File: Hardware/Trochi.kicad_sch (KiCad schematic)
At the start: 49 parts, among them IC1 ICM-42688-P, J1 JST PH, J2 JST-SH, J3 JST-SH, J4 JST-SH, J5 JST-SH, J6 JST_SH, Q1 AO3400A, Q2 AO3400A, Q3 AO3400A, Q4 AO3400A, Q5 AO3400A, SW1 SW_SPDT, U1 ME6211C33M5, U2 YX-SMD5020

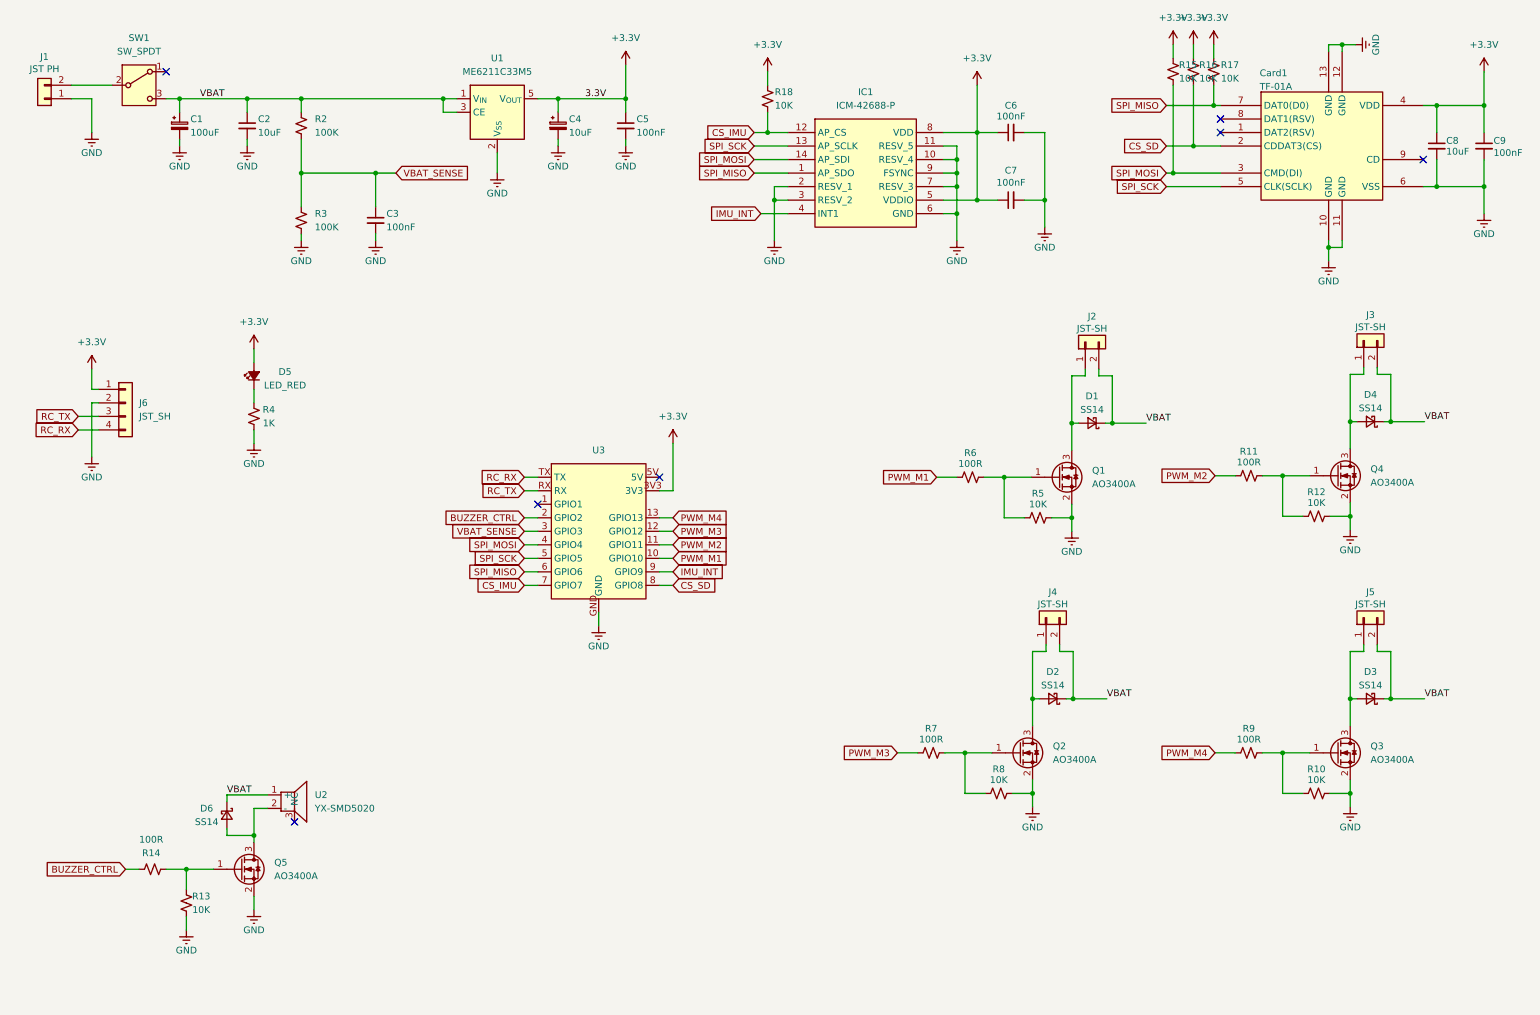
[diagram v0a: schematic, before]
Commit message: style: organize and finalize schematic layout
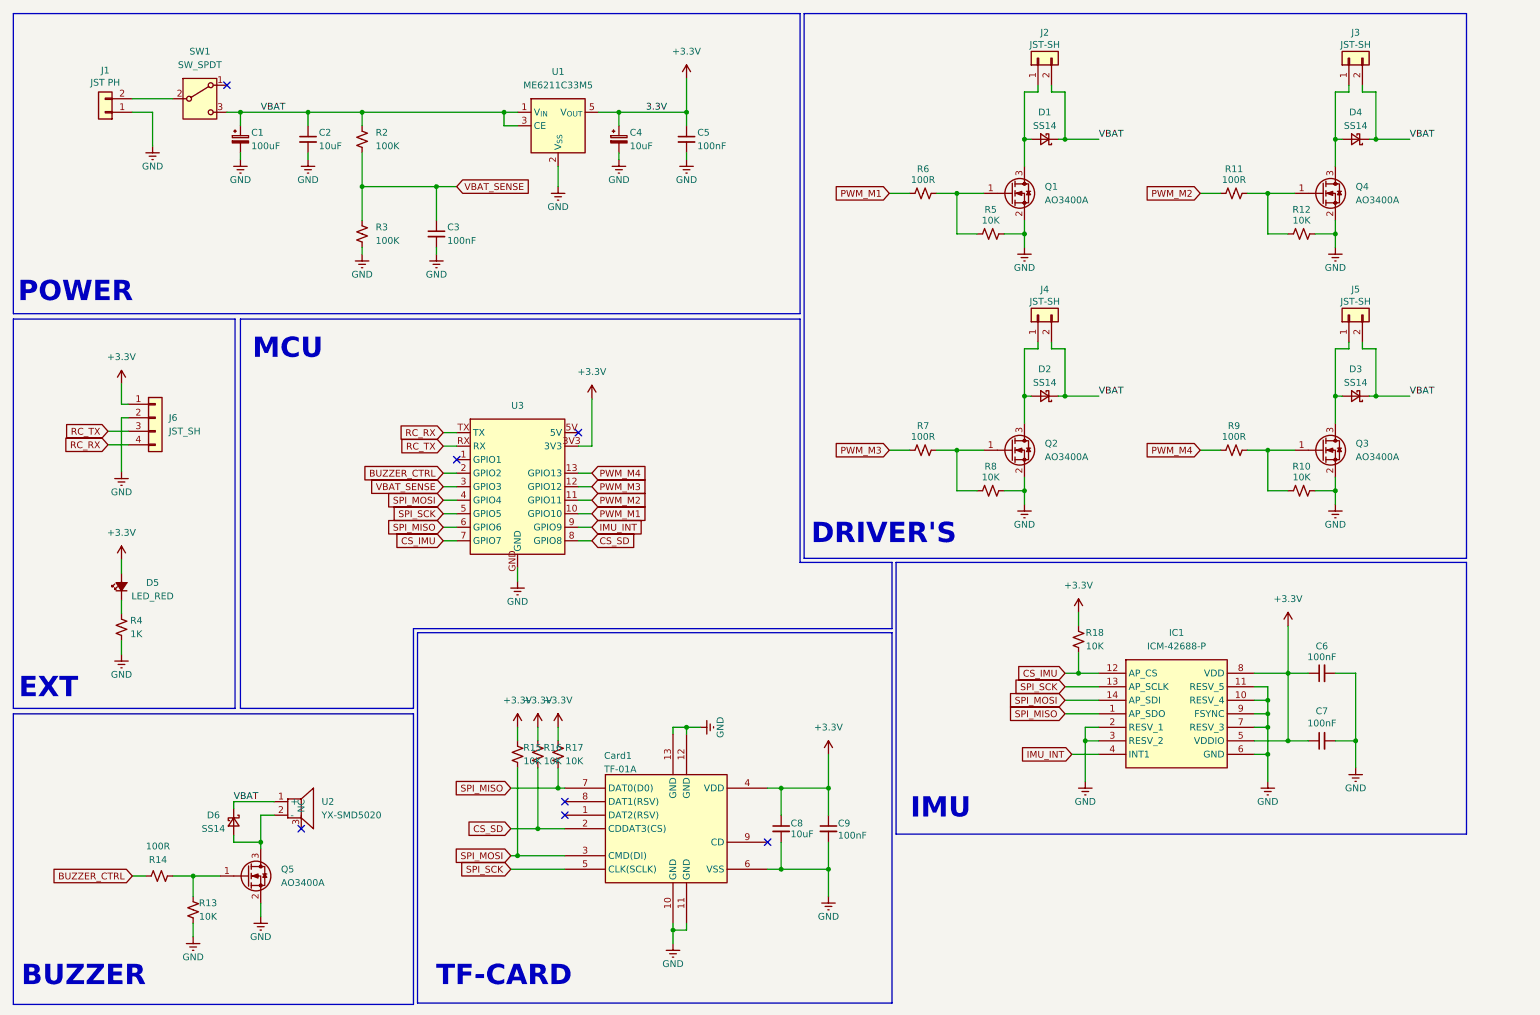
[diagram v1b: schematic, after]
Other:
- note added: "BUZZER"
- note added: "DRIVER'S"
- note added: "EXT"
- note added: "IMU"
- note added: "MCU"
- note added: "POWER"
- note added: "TF-CARD"
- moved on the sheet: C1, C2, C3, C4, C5, C6, C7, C8, C9, Card1, D1, D2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
